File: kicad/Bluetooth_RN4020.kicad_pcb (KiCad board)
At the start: 2 copper layers, 86.4 x 61 mm, 15 parts, among them P1 CONN_5, P2 CONN_4, U1 RN4020

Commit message: Poncho Mediano
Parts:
- removed G***: Logo_EDU-CIAA, Poncho_Esqueleto:Logo_EDU-CIAA
- removed G***: LOGO, Poncho_Esqueleto:Logo_Poncho
- removed G101: Logo_OSHWA, Poncho_Esqueleto:Logo_OSHWA
- removed MP?: Plantilla_EDU-CIAA, Poncho_Esqueleto:Plantilla_EDU-CIAA
- removed P1: CONN_5, Poncho_Modelos:bornier5
- removed P2: CONN_4, Poncho_Modelos:bornier4
- XA1: footprint Poncho_Esqueleto:Conn_Poncho_Chico -> Poncho_Esqueleto:Conn_Poncho_Mediano
- moved XA1 269.9 mm to (185.2, 64.0)
- moved D1 51.8 mm to (169.4, 96.1), turned to 270 degrees
- moved R1 48.1 mm to (169.5, 110.2), turned to 90 degrees
- moved C1 47.8 mm to (140.5, 131.2)
- moved U1 42.2 mm to (156.1, 123.2), turned to 180 degrees
- moved D2 40.5 mm to (163.0, 96.1), turned to 270 degrees
- moved R2 35.6 mm to (163.1, 110.2), turned to 90 degrees
- moved D3 30.4 mm to (156.7, 96.1), turned to 270 degrees
- moved R3 23.6 mm to (156.9, 110.2), turned to 90 degrees
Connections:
- U1 pad 13: (no net) -> N-000004
- U1 pad 14: (no net) -> CTS
- U1 pad 15: (no net) -> HW
- U1 pad 17: (no net) -> N-000005
- U1 pad 18: (no net) -> RTS
- U1 pad 19: (no net) -> N-000006
- U1 pad 2: (no net) -> N-000001
- U1 pad 20: (no net) -> N-0000024
- U1 pad 21: (no net) -> N-0000023
- U1 pad 22: (no net) -> N-0000022
- U1 pad 3: (no net) -> N-000002
- U1 pad 4: (no net) -> N-000003
- U1 pad 5: (no net) -> UART_TX
- U1 pad 6: (no net) -> UART_RX
- U1 pad 7: (no net) -> SW
- U1 pad 8: (no net) -> CMD
- XA1 pad 44: (no net) -> Net-(P2-Pad3)
- XA1 pad 56: (no net) -> Net-(P2-Pad2)
- XA1 pad 72: Net-(P2-Pad3) -> (no net)
- XA1 pad 74: Net-(P2-Pad2) -> (no net)
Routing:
- net GND: track 155.8 -> 20.9 mm
- net +5VP: track 73.3 -> 0.00 mm
- net Net-(P1-Pad4): track 60.1 -> 0.00 mm
- net Net-(P1-Pad3): track 54.7 -> 0.00 mm
- net Net-(P2-Pad3): track 43.4 -> 0.00 mm
- net +3.3V: track 45.2 -> 4.34 mm
- net Net-(P2-Pad2): track 36.9 -> 0.00 mm
- net +5V: track 28.8 -> 0.00 mm
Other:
- board outline removed
- net class Default: clearance 0.508 -> 0.25
- rule trace_clearance: 0.508 -> 0.25
- board text removed: "Borrar (Footprint MP1) la Plantilla-EDU-CIAA al finalizar el posicionamiento y definido el borde de PCB."
- board text removed: "Diseño simple faz. Sin requerimientos especiales."
- board text removed: "Editar el rótulo"
- board text removed: "Editar el stackup para reflejar cantidad de capas, si se han realizado cálculos de impedancia o si es relevante para el funcionamiento."
- board text removed: "PONCHO CHICO"
- board text removed: "PONCHO CHICO http://www.proyecto-ciaa.com.ar/"
- board text removed: "Para un diseño nuevo luego de modificar el esquemático: 1)Seleccionar el bloque del PCB y cotas. (click-drag-release). 2)Opción de borrar bloque (Botón derecho). 3)Marcar todo menos locked footprints (MP1 y XA1) 4) Aceptar. 5) Volver a cargar el netlist."
- board text removed: "STACK-UP"
- board text removed: "Se sugiere colocar código de Poncho en cobre, serigrafía y rótulo."
- board text removed: "www.proyecto-ciaa.com.ar"

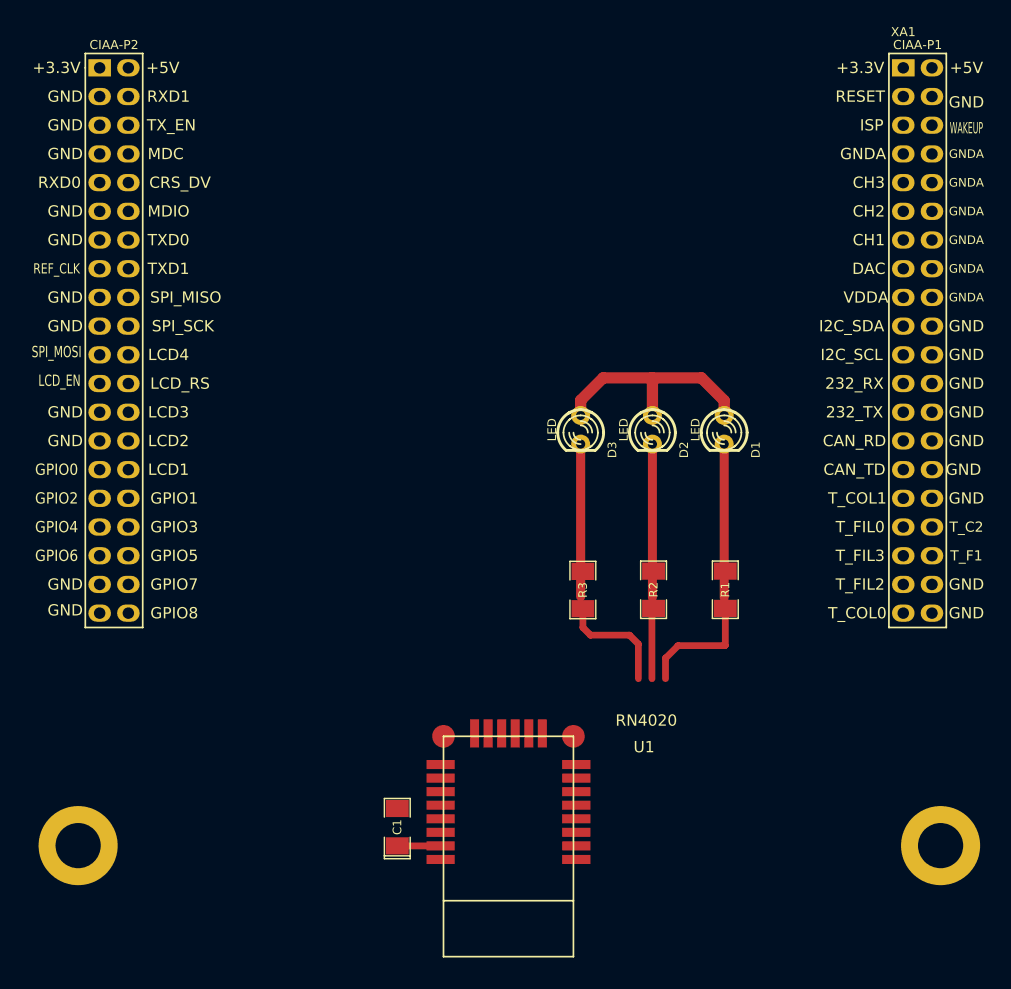
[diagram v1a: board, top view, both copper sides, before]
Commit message: 50% Poncho
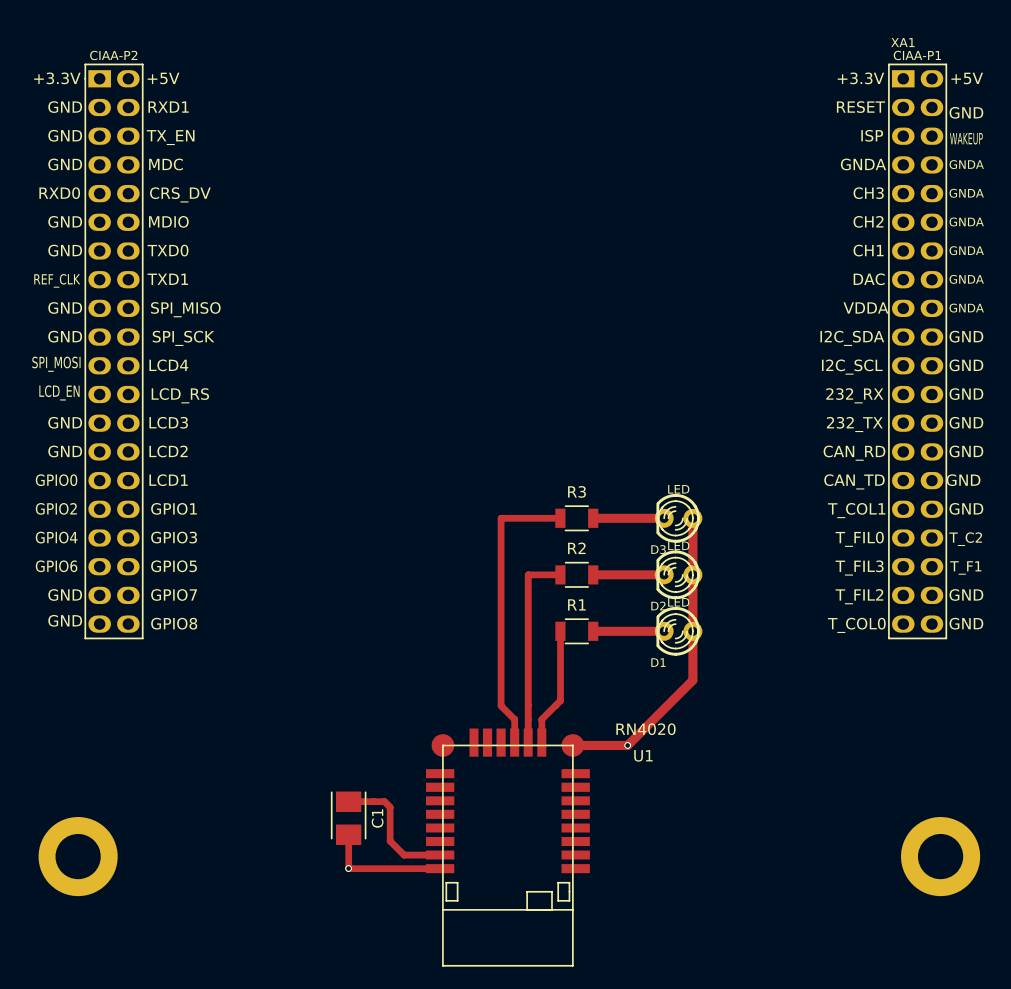
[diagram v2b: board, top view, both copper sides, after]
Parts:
- C1: footprint SM1206POL -> Capacitors_Tantalum_SMD:TantalC_SizeB_EIA-3528_Reflow
- R1, R2, R3: footprint SM1206 -> Resistors_SMD:R_1206
- moved D1 18.3 mm to (165.4, 113.9), turned to 180 degrees
- moved R1 13.6 mm to (156.4, 113.9), turned to 0 degrees
- moved D2 13.0 mm to (165.4, 108.9), turned to 180 degrees
- moved D3 11.7 mm to (165.4, 103.9), turned to 180 degrees
- moved R2 6.92 mm to (156.4, 108.9), turned to 0 degrees
- moved R3 6.37 mm to (156.4, 103.9), turned to 0 degrees
- moved C1 4.38 mm to (136.2, 130.4), turned to 270 degrees
- moved XA1 0.97 mm to (185.2, 65.0)
- moved U1 0.81 mm to (156.0, 124.0)
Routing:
- net GND: track 20.9 -> 38.5 mm, vias 0 -> 2
- net N-0000019: track 10.3 -> 25.6 mm
- net N-000007: track 6.47 -> 17.7 mm
- net +3.3V: track 4.34 -> 11.8 mm
- net N-0000018: track 13.7 -> 6.28 mm
- net N-0000017: track 13.6 -> 6.28 mm
- net N-0000016: track 13.6 -> 6.28 mm
